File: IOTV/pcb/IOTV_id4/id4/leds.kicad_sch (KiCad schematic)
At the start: 50 parts, among them Q1 S8050, Q10 S8050, Q11 S8050, Q12 S8050, Q2 S8050, Q3 S8050, Q7 S8050, Q8 S8050, Q9 S8050

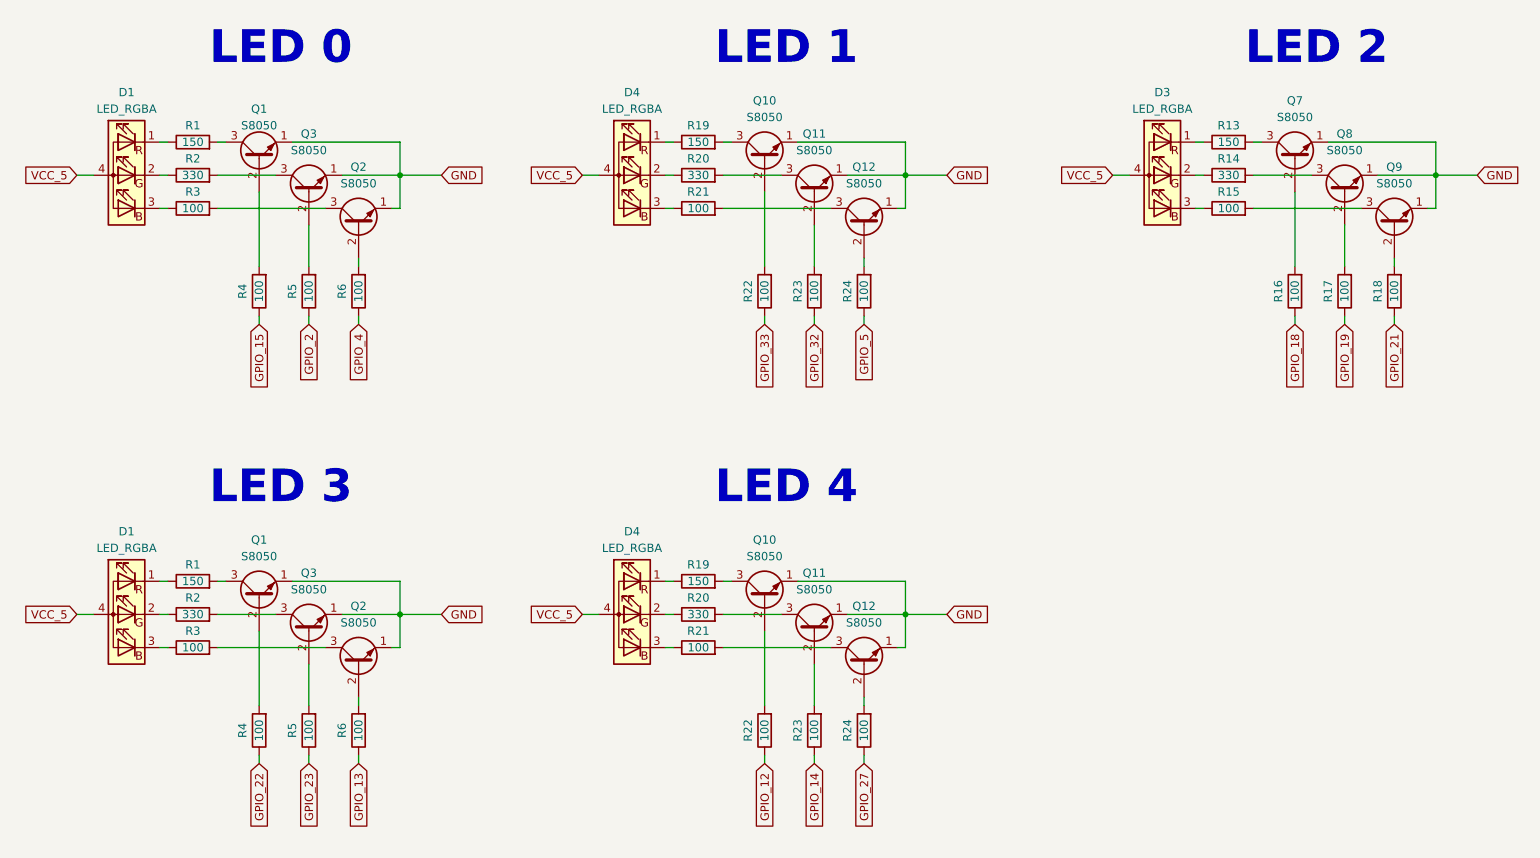
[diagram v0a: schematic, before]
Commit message: PCB - ID4
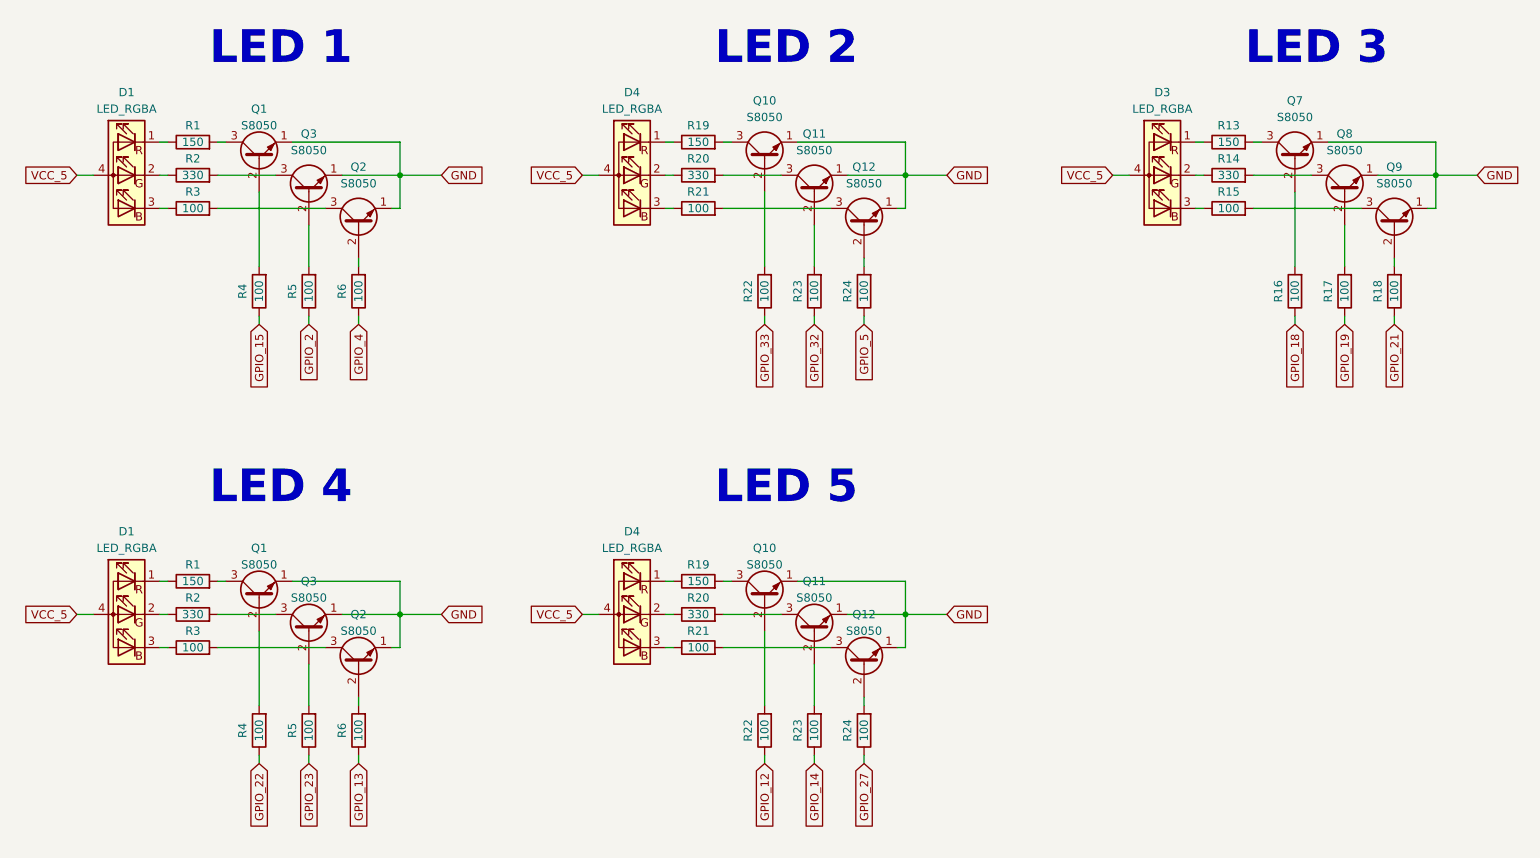
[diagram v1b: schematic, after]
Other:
- note added: "LED 5"
- note removed: "LED 0"
